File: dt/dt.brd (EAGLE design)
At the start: 148.6 x 101.6 mm, 265 parts, among them IC1 TL072D, IC10 LM317, IC11 LM337, IC2 TL072D, IC3 TL072D, IC4 TL072D, IC5 TL072D, IC6 TL072D, IC7 AT45DB161D-SU, U1 LM1117DTX-3.3, U2 PCN2-S5-D12-S, U3 STM32F7X3ZXT, U4 USBLC6-2SC6YSOT23-6L_STM-M, U5 USBLC6-2SC6YSOT23-6L_STM-M, U6 PCM1681PWPPWP28_6P46X2P4-M, U7 PCM1681PWPPWP28_6P46X2P4-M, Y1 ABLS7M2-25.000MHZ-D2Y-T

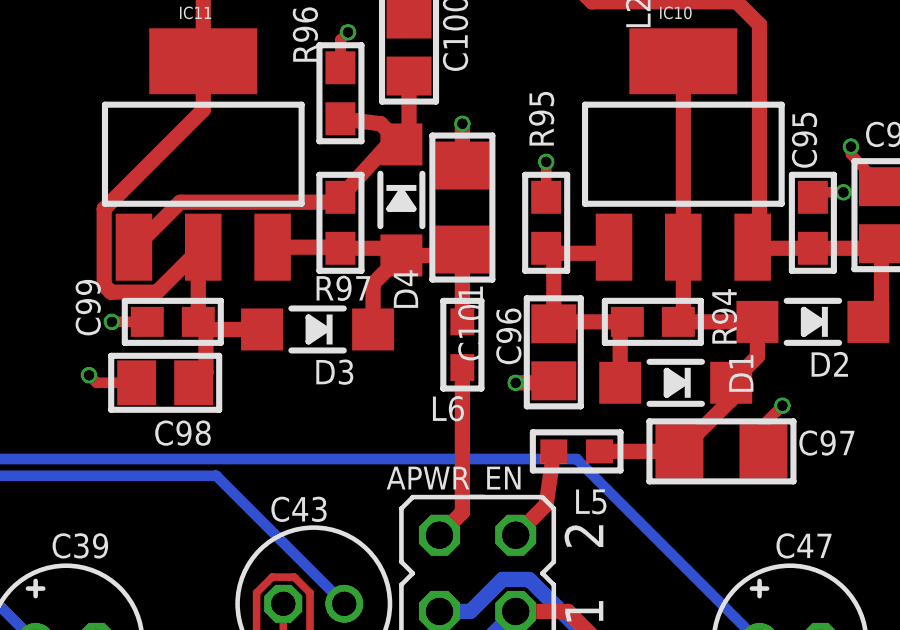
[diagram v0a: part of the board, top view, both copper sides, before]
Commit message: wip
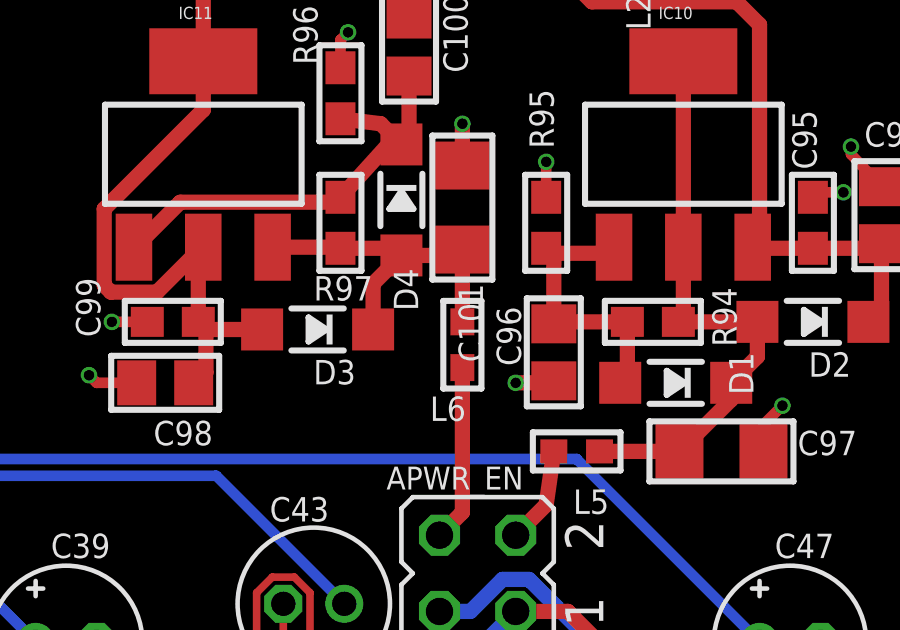
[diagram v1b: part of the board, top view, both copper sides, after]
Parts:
- C101, C97: value 1uF 12065C105M4Z2A -> 1u 12065C105M4Z2A
- C75: value 4.7uF -> 4.7u
- C80, C84, C85, C86, C90, C91: value 1uF Ceramic -> 1u Ceramic
- C81, C82, C83, C87, C88, C89, C92, C93: value 10uF Electrolyte -> 10u Electrolyte
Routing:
- net N$73: track 10.3 -> 9.65 mm
